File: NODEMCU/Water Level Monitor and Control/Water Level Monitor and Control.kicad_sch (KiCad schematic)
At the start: 52 parts, among them J1 PUMP, J2 12VAC_IN, K1 10A RELAY, U1 LM2596S-5V, U2 HC-SR04, U6 PCA9555D

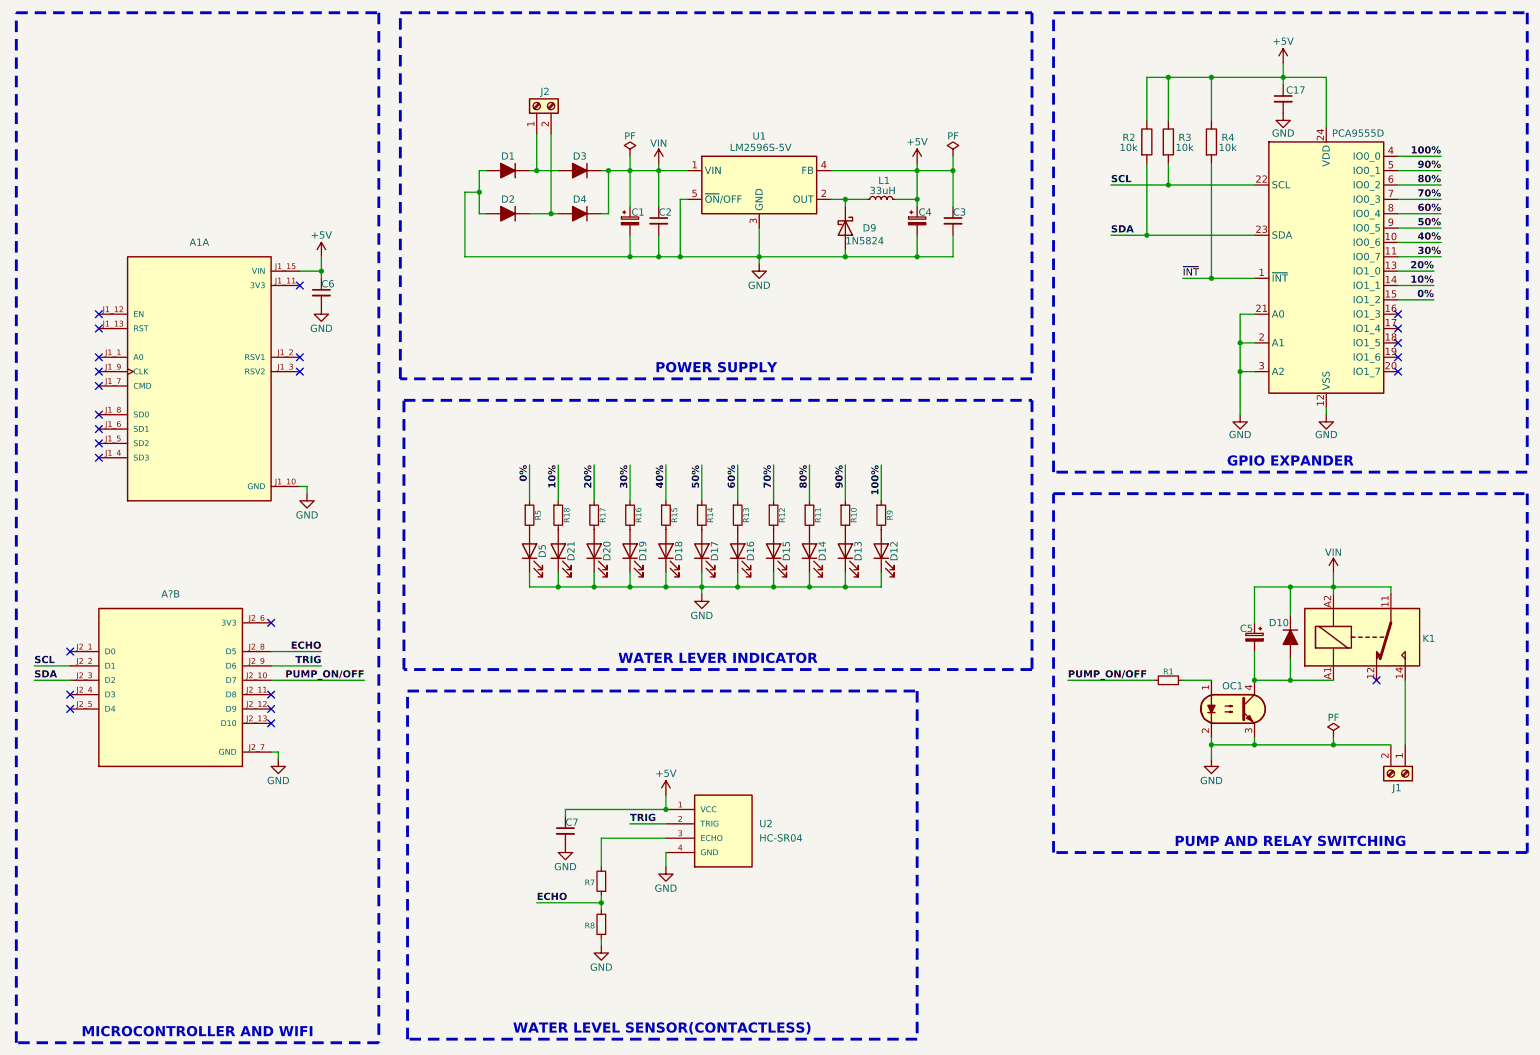
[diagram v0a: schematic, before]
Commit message: update from work
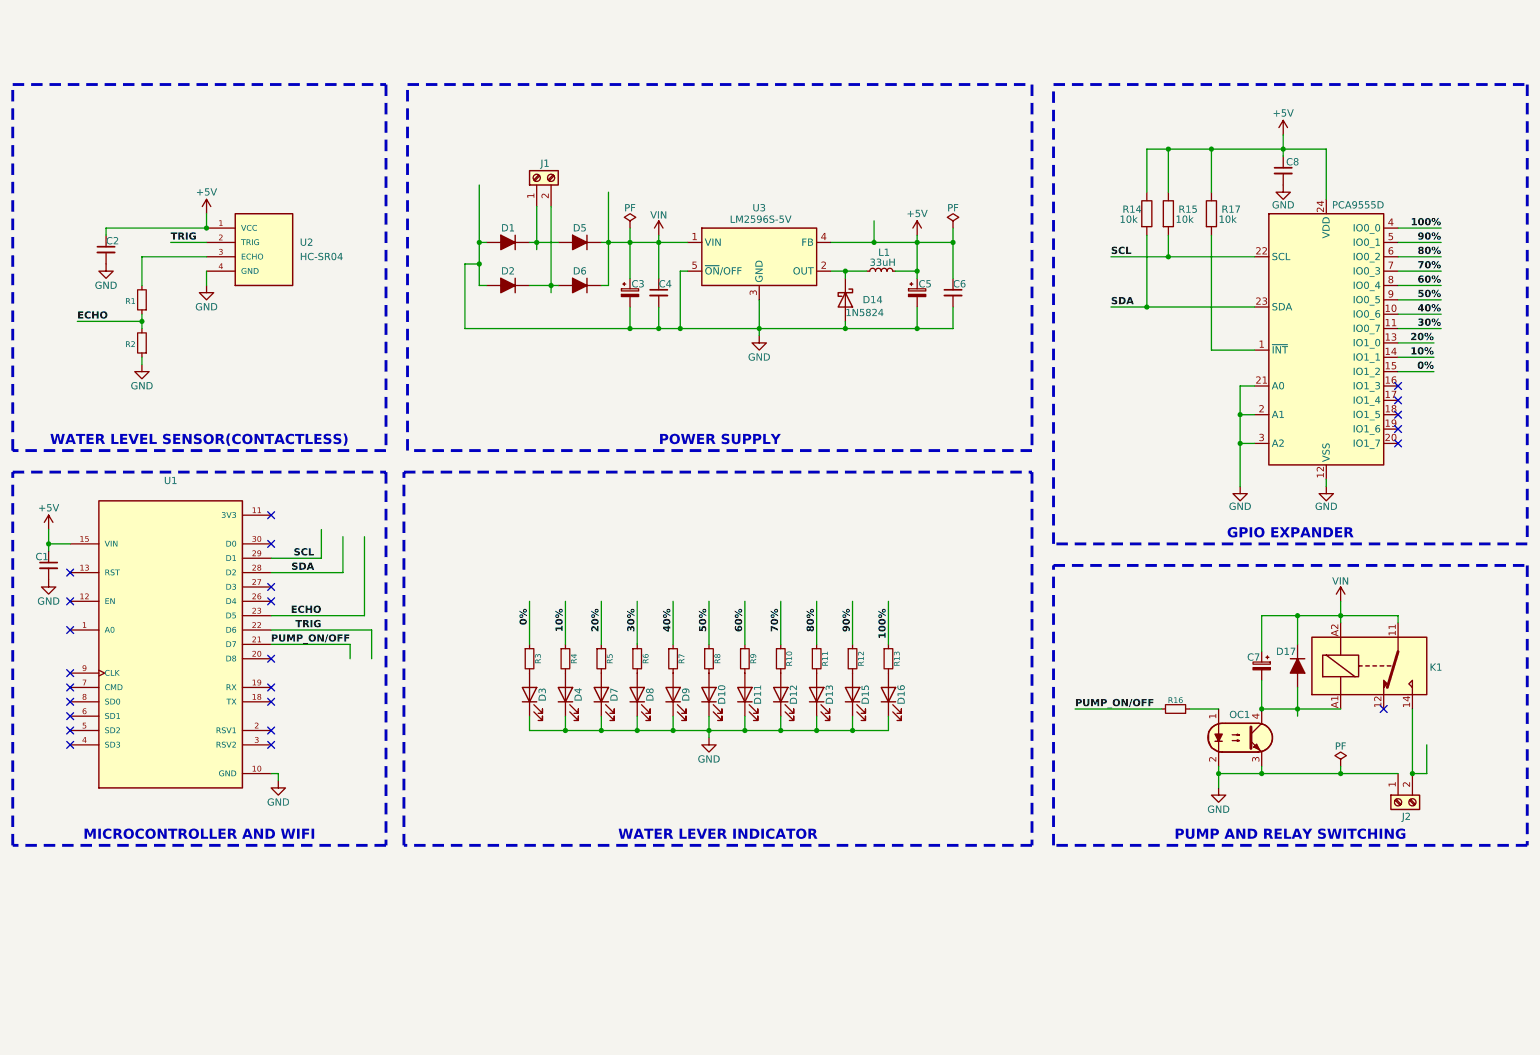
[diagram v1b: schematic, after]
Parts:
- removed A1: Nodemcu_Side B, 113990105:SEEED_113990105, symbol nodemcu:113990105
- removed A?: Nodemcu, 113990105:SEEED_113990105, symbol nodemcu:113990105
- removed C6: 100nF, symbol Device:C_Small
- added C1: 100nF, Capacitor_THT:C_Disc_D5.1mm_W3.2mm_P5.00mm, symbol Device:C_Small
- added U1: ESP8266 NODEMCU, Footprint:nodemcu, symbol nodemcu:ZC563900
- C2: renamed from C7; footprint (none) -> Capacitor_THT:C_Disc_D5.1mm_W3.2mm_P5.00mm
- C3: renamed from C1; footprint (none) -> Capacitor_THT:CP_Radial_D18.0mm_P7.50mm
- C4: renamed from C2; footprint (none) -> Capacitor_THT:C_Disc_D5.1mm_W3.2mm_P5.00mm
- C5: renamed from C4; footprint (none) -> Capacitor_THT:CP_Radial_D8.0mm_P3.80mm
- C6: renamed from C3; footprint (none) -> Capacitor_THT:C_Disc_D5.1mm_W3.2mm_P5.00mm
- C7: renamed from C5; footprint (none) -> Capacitor_THT:CP_Radial_D5.0mm_P2.50mm
- C8: renamed from C17; footprint PCM_JLCPCB:C_0805 -> Capacitor_THT:C_Disc_D5.1mm_W3.2mm_P5.00mm
- D1, D2: footprint PCM_Diode_THT_AKL:D_DO-41_SOD81_P7.62mm_Horizontal -> Diode_THT:D_A-405_P10.16mm_Horizontal
- D10: renamed from D17; footprint (none) -> LED_THT:LED_D5.0mm
- D11: renamed from D16; footprint (none) -> LED_THT:LED_D5.0mm
- D12: renamed from D15; footprint (none) -> LED_THT:LED_D5.0mm
- D13: renamed from D14; footprint (none) -> LED_THT:LED_D5.0mm
- D14: renamed from D9; footprint Diode_THT:D_DO-201AD_P15.24mm_Horizontal -> Diode_SMD:D_2010_5025Metric
- D15: renamed from D13; footprint (none) -> LED_THT:LED_D5.0mm
- D16: renamed from D12; footprint (none) -> LED_THT:LED_D5.0mm
- D17: renamed from D10; footprint PCM_Diode_THT_AKL:D_DO-41_SOD81_P7.62mm_Horizontal -> Diode_THT:D_A-405_P10.16mm_Horizontal
- D3: renamed from D5; footprint (none) -> LED_THT:LED_D5.0mm
- D4: renamed from D21; footprint (none) -> LED_THT:LED_D5.0mm
- D5: renamed from D3; footprint PCM_Diode_THT_AKL:D_DO-41_SOD81_P7.62mm_Horizontal -> Diode_THT:D_A-405_P10.16mm_Horizontal
- D6: renamed from D4; footprint PCM_Diode_THT_AKL:D_DO-41_SOD81_P7.62mm_Horizontal -> Diode_THT:D_A-405_P10.16mm_Horizontal
- D7: renamed from D20; footprint (none) -> LED_THT:LED_D5.0mm
- D8: renamed from D19; footprint (none) -> LED_THT:LED_D5.0mm
- D9: renamed from D18; footprint (none) -> LED_THT:LED_D5.0mm
- L1: footprint (none) -> Inductor_SMD:L_12x12mm_H4.5mm
- R1: renamed from R7; footprint (none) -> Resistor_THT:R_Axial_DIN0207_L6.3mm_D2.5mm_P7.62mm_Horizontal
- R10: renamed from R12; footprint (none) -> Resistor_THT:R_Axial_DIN0207_L6.3mm_D2.5mm_P7.62mm_Horizontal
- R11: footprint (none) -> Resistor_THT:R_Axial_DIN0207_L6.3mm_D2.5mm_P7.62mm_Horizontal
- R12: renamed from R10; footprint (none) -> Resistor_THT:R_Axial_DIN0207_L6.3mm_D2.5mm_P7.62mm_Horizontal
- R13: renamed from R9; footprint (none) -> Resistor_THT:R_Axial_DIN0207_L6.3mm_D2.5mm_P7.62mm_Horizontal
- R14: renamed from R2; footprint PCM_JLCPCB:R_0805 -> Resistor_THT:R_Axial_DIN0207_L6.3mm_D2.5mm_P7.62mm_Horizontal
- R15: renamed from R3; footprint PCM_JLCPCB:R_0805 -> Resistor_THT:R_Axial_DIN0207_L6.3mm_D2.5mm_P7.62mm_Horizontal
- R16: renamed from R1; footprint (none) -> Resistor_THT:R_Axial_DIN0207_L6.3mm_D2.5mm_P7.62mm_Horizontal
- R17: renamed from R4; footprint PCM_JLCPCB:R_0805 -> Resistor_THT:R_Axial_DIN0207_L6.3mm_D2.5mm_P7.62mm_Horizontal
- R2: renamed from R8; footprint (none) -> Resistor_THT:R_Axial_DIN0207_L6.3mm_D2.5mm_P7.62mm_Horizontal
- R3: renamed from R5; value 330 -> 220; footprint (none) -> Resistor_THT:R_Axial_DIN0207_L6.3mm_D2.5mm_P7.62mm_Horizontal
- R4: renamed from R18; value 330 -> 220; footprint (none) -> Resistor_THT:R_Axial_DIN0207_L6.3mm_D2.5mm_P7.62mm_Horizontal
- R5: renamed from R17; footprint (none) -> Resistor_THT:R_Axial_DIN0207_L6.3mm_D2.5mm_P7.62mm_Horizontal
- R6: renamed from R16; footprint (none) -> Resistor_THT:R_Axial_DIN0207_L6.3mm_D2.5mm_P7.62mm_Horizontal
- R7: renamed from R15; footprint (none) -> Resistor_THT:R_Axial_DIN0207_L6.3mm_D2.5mm_P7.62mm_Horizontal
- R8: renamed from R14; footprint (none) -> Resistor_THT:R_Axial_DIN0207_L6.3mm_D2.5mm_P7.62mm_Horizontal
- R9: renamed from R13; footprint (none) -> Resistor_THT:R_Axial_DIN0207_L6.3mm_D2.5mm_P7.62mm_Horizontal
- U2: footprint HC-SR04:XCVR_HC-SR04 -> Footprint:XCVR_HC-SR04
- renumbered J2 to J1, J1 to J2, U1 to U3, U6 to U4
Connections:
- net +5V: now also C1.1, U1.15 (VIN)
- net 3V3: now also U1.11 (3V3), U1.16 (3V3), U1.25 (3V3)
- net ECHO: now also U1.23 (D5)
- net GND: now also J2.1 (Pin_1), C1.2, U1.10 (GND), U1.14 (GND), U1.17 (GND), U1.24 (GND); no longer J2.2 (Pin_2)
- net PUMP_ON/OFF: now also U1.21 (D7)
- net SCL: now also U1.29 (D1)
- net SDA: now also U1.28 (D2)
- net TRIG: now also U1.22 (D6)
- net at K1.14: now also J2.2 (Pin_2); no longer J2.1 (Pin_1)
- net ~{INT}: no longer names the net of R17.1, U4.1 (~{INT})
- no-connect marks 25 -> 24
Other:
- moved on the sheet: C2, C3, C4, C5, C6, C7, C8, D1, D10, D11, D12, D13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
